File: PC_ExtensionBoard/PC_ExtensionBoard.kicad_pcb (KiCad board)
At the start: 2 copper layers, 135 x 125 mm, 2 parts, among them CN1 QT002206-4131-3H, CN2 QT002206-4131-3H

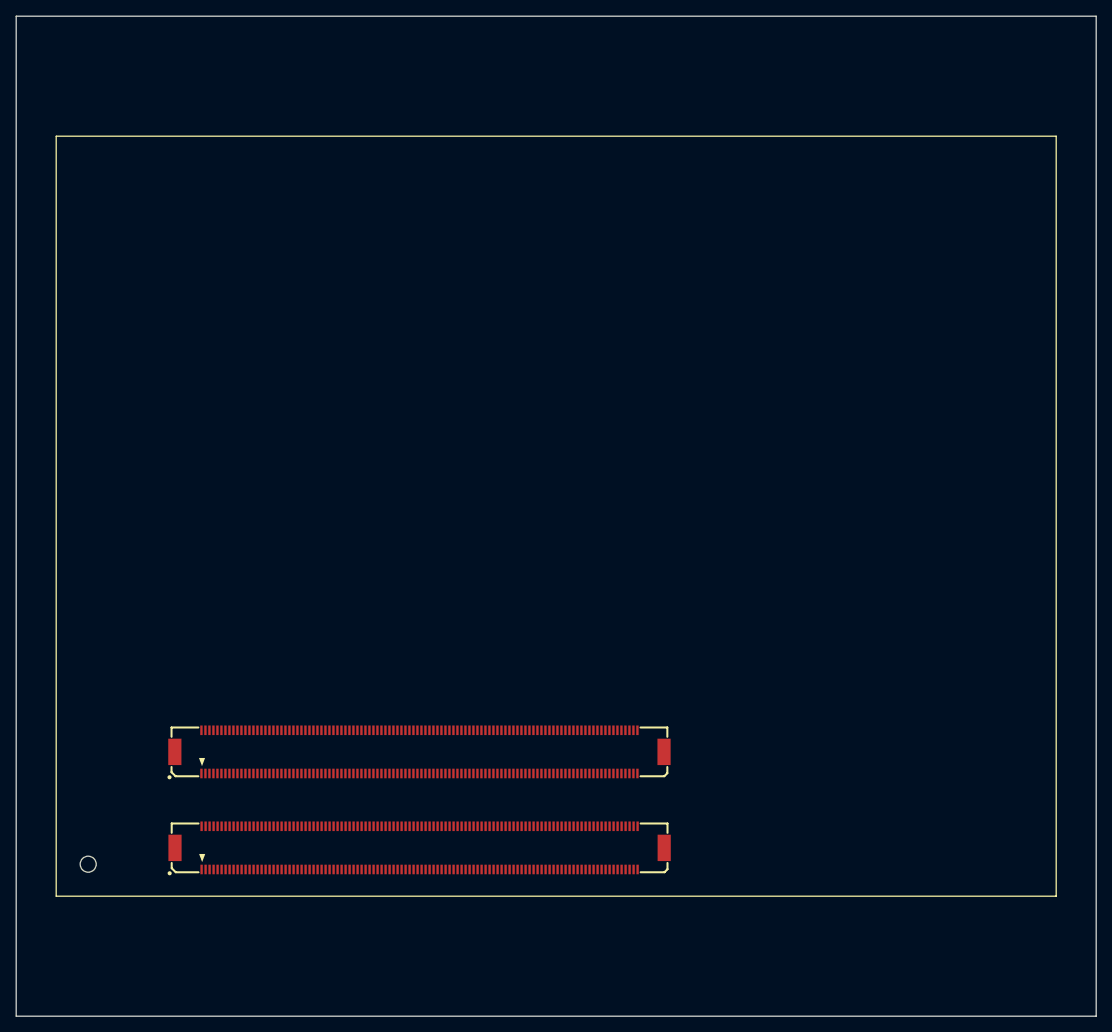
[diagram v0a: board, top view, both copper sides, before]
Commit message: update 3d
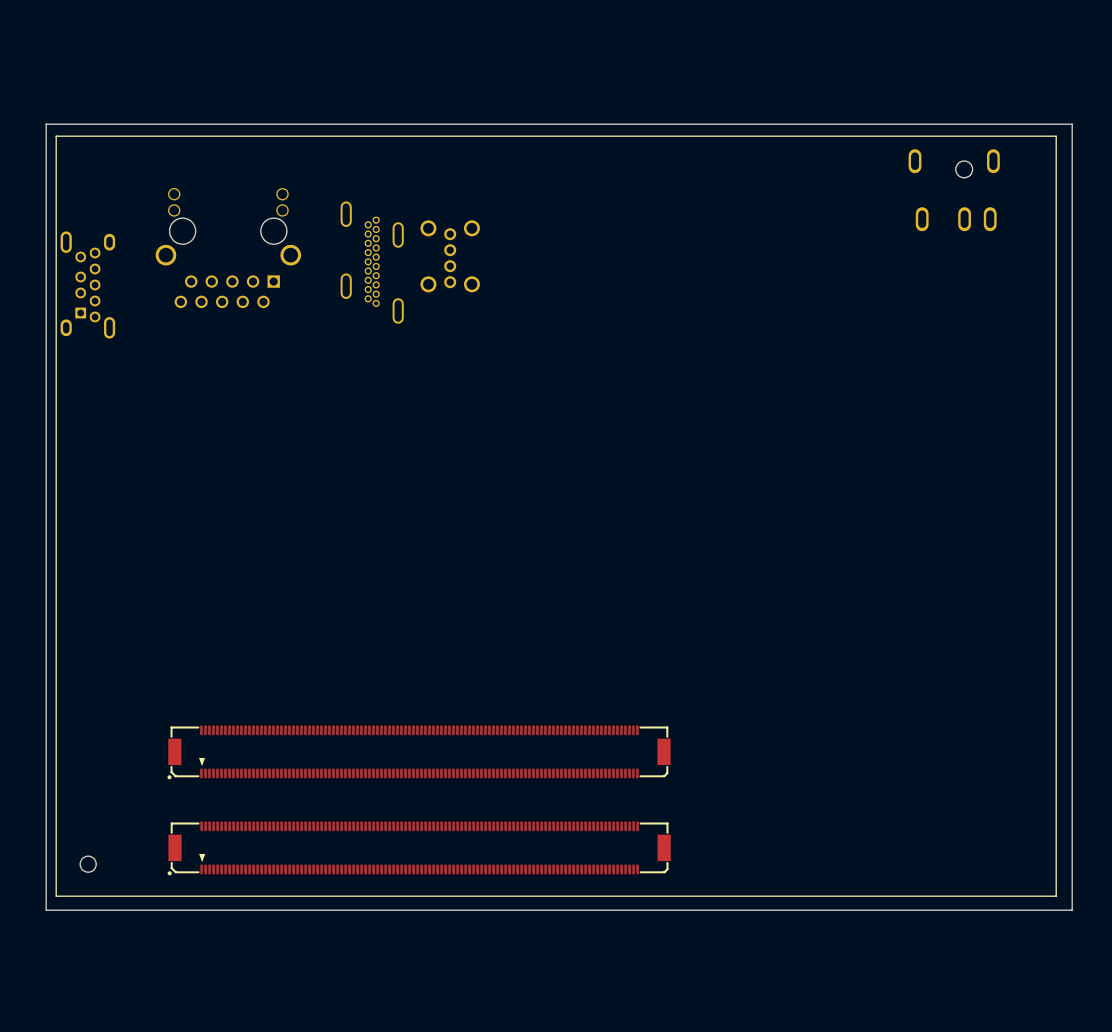
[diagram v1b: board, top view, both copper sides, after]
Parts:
- added CN3: HYC70-HDMIA19-230, DatCao_FootPrint:HDMI-TH_HYC70-HDMIA19-230, B.Cu at (89.5, 65.8)
- added DC1: DC-044A-20A, DatCao_FootPrint:DC-IN-TH_DC-044A-20A, B.Cu at (162.2, 56.8)
- added RJ1: 936273608, DatCao_FootPrint:RJ45-TH_936273608, B.Cu at (71.5, 64.0)
- added USB1: HC-USB3.0-L257-J, DatCao_FootPrint:USB-A-TH_HC-USB3.0-L257-J, B.Cu at (54.0, 68.6)
- added USB2: HC-USB2.0-L195-P, DatCao_FootPrint:USB-TH_73725-0110BLF, B.Cu at (99.2, 65.0)
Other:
- board size 135 x 125 mm -> 128.2 x 98.2 mm
